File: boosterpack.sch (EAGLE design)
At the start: 25 parts, among them J1 POWERPOLE_DOUBLE

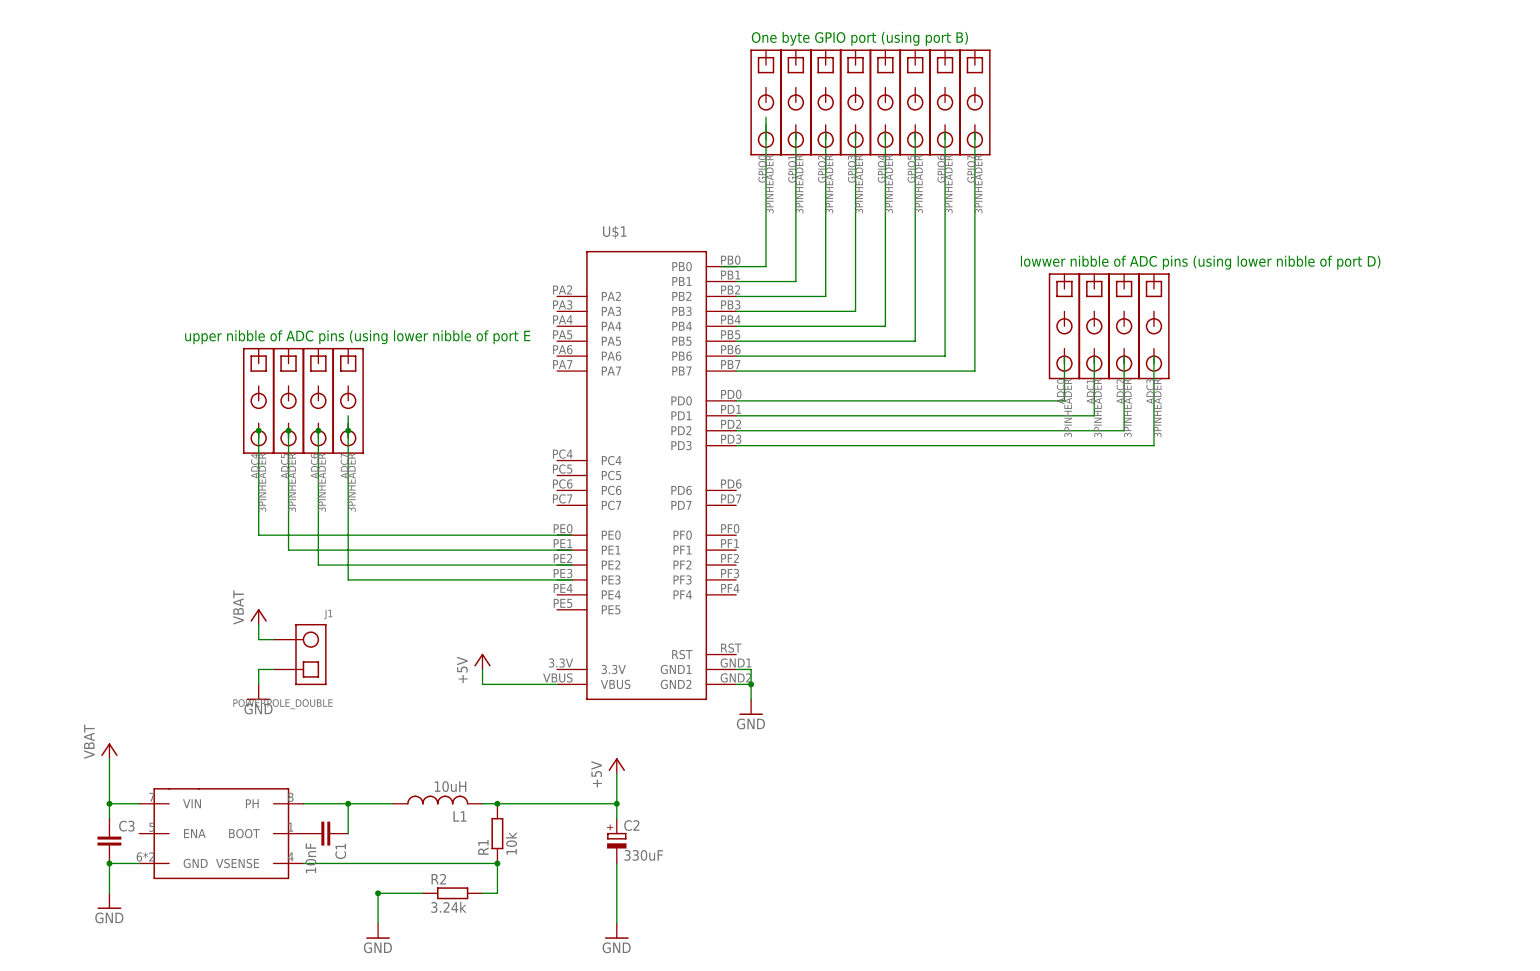
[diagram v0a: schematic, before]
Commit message: lots of routing; moustly just routing
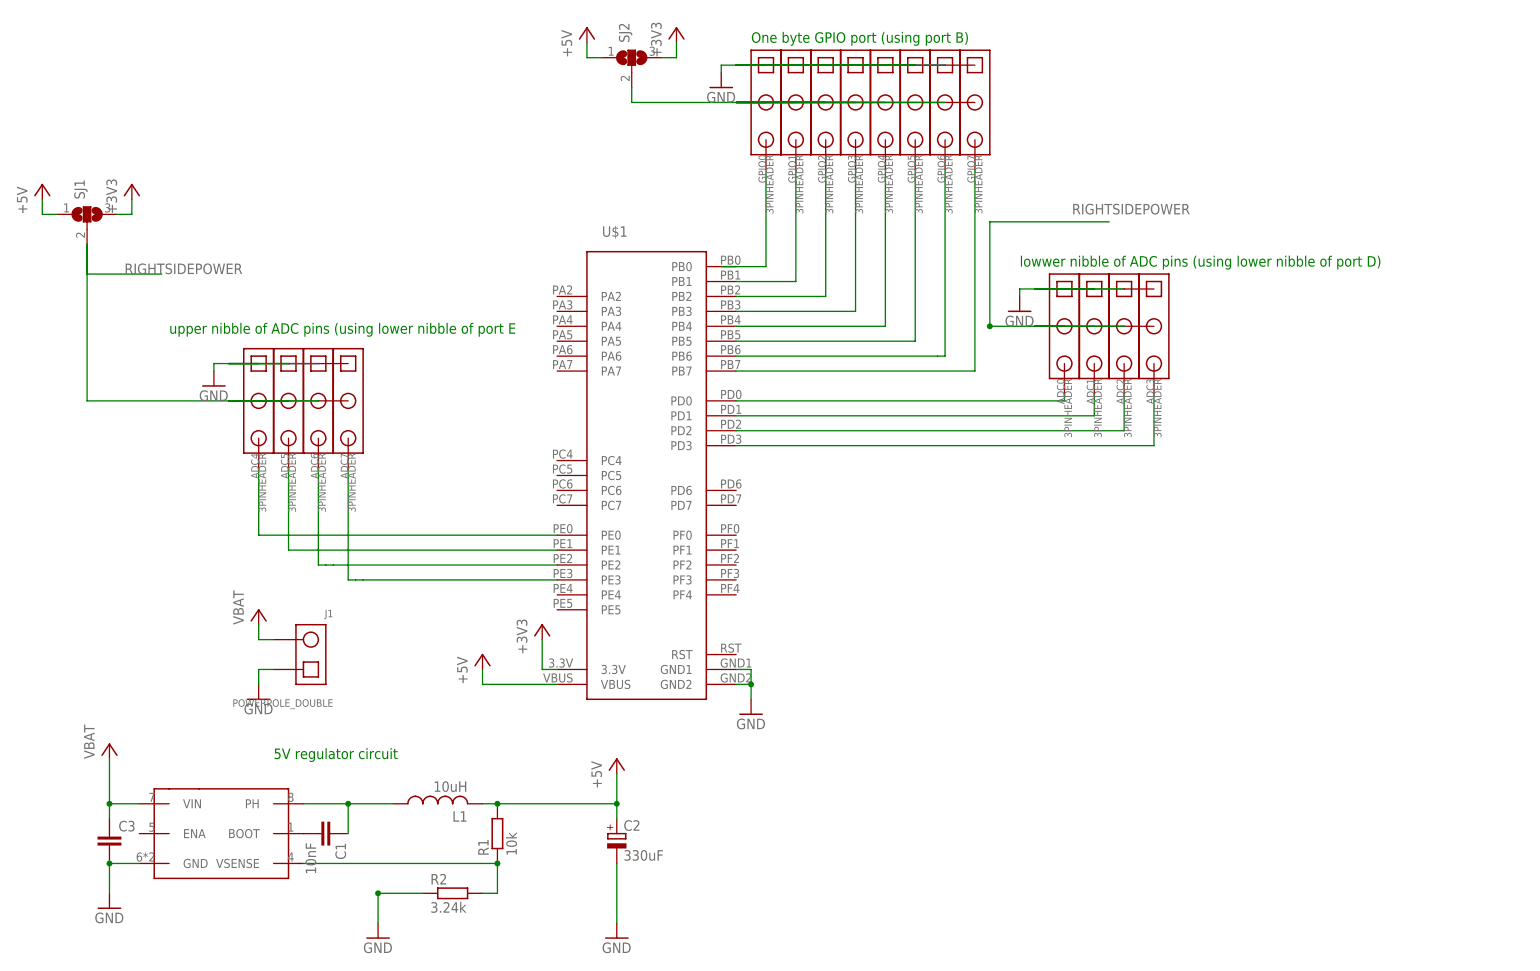
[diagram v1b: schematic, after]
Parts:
- added SJ1, SJ2: (no value), jumper:SJ2W
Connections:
- new net ADC5: ADC5.3, U$1.PE1
- new net N$13: ADC4.3, U$1.PE0
- new net N$16: SJ1.3, SJ2.3, U$1.3.3V
- new net N$4: ADC6.3, U$1.PE2
- new net N$5: ADC7.3, U$1.PE3
- new net RIGHTSIDEPOWER: ADC0.2, ADC1.2, ADC2.2, ADC3.2, ADC4.2, ADC5.2, ADC6.2, ADC7.2, SJ1.2
- net +5V: now also SJ1.1, SJ2.1
- net ADC1: now also ADC1.3
- net ADC2: now also ADC2.3
- net ADC3: now also ADC3.3
- net GND: now also ADC0.1, ADC1.1, ADC2.1, ADC3.1, ADC4.1, ADC5.1, ADC6.1, ADC7.1, GPIO0.1, GPIO1.1, GPIO2.1, GPIO3.1, GPIO4.1, GPIO5.1, GPIO6.1, GPIO7.1
- net GPIO0: now also GPIO0.3
- net GPIO1: now also GPIO1.3
- net GPIO2: now also GPIO2.3
- net GPIO3: now also GPIO3.3
- net N$1: now also ADC0.3
- net N$2: now also GPIO4.3
- net N$3: now also GPIO5.3
- net N$6: now also GPIO6.3
- net N$7: now also GPIO0.2, GPIO1.2, GPIO2.2, GPIO3.2, GPIO4.2, GPIO5.2, GPIO6.2, GPIO7.2, SJ2.2; no longer GPIO0.1
- net N$8: now also GPIO7.3
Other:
- note added: "5V regulator circuit"
- moved on the sheet: ADC0, ADC1, ADC2, ADC3, ADC4, ADC5, ADC6, ADC7, GPIO0, GPIO1, GPIO2, GPIO3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
